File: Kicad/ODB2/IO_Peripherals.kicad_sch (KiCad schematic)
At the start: 23 parts, among them J1 Cam_Conn_01x01_Socket, J5 RFM_Conn_Coaxial, U10 W25Q512JVEIQ

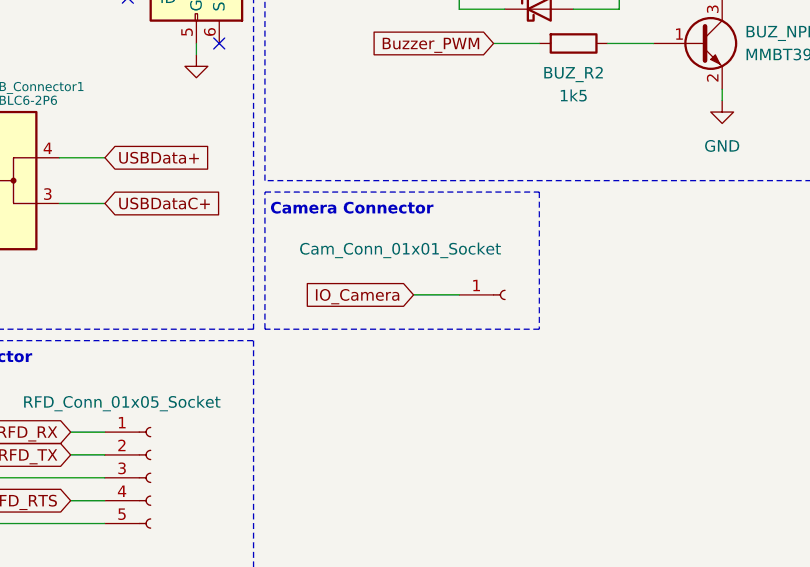
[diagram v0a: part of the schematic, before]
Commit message: fix my shit (cam io)
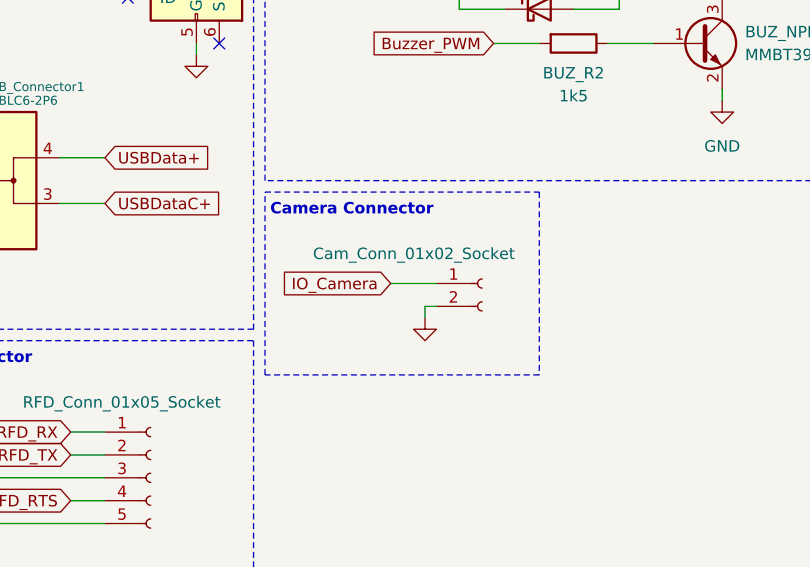
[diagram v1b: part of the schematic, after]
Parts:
- removed J1: Cam_Conn_01x01_Socket, Connector_PinHeader_2.00mm:PinHeader_1x01_P2.00mm_Vertical, symbol Connector:Conn_01x01_Socket
- added J1: Cam_Conn_01x02_Socket, Connector_PinHeader_2.00mm:PinHeader_1x02_P2.00mm_Vertical, symbol Connector:Conn_01x02_Socket
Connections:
- net GND: now also J1.2 (Pin_2)
- net IO_Camera: now also J1.1 (Pin_1)
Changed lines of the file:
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@@
 	(wire
 		(pts
+			(xy 124.46 76.2) (xy 123.19 76.2)
+		)
+		(stroke
+			(width 0)
+			(type default)
+		)
+	)
+	(wire
+		(pts
 			(xy 54.61 119.38) (xy 54.61 120.65)
 		)
@@
 	(wire
 		(pts
+			(xy 123.19 76.2) (xy 123.19 77.47)
+		)
+		(stroke
+			(width 0)
+			(type default)
+		)
+	)
+	(wire
+		(pts
 			(xy 64.77 95.25) (xy 87.63 95.25)
 		)
@@
 	(wire
 		(pts
-			(xy 121.92 74.93) (xy 127 74.93)
+			(xy 119.38 73.66) (xy 124.46 73.66)
 		)
 		(stroke
@@
 	(rectangle
 		(start 105.41 63.5)
-		(end 135.89 78.74)
+		(end 135.89 83.82)
 		(stroke
 			(width 0)
@@
 	(global_label "IO_Camera"
 		(shape input)
-		(at 121.92 74.93 180)
+		(at 119.38 73.66 180)
 		(fields_autoplaced yes)
 		(effects
@@
 		)
 		(property "Intersheetrefs" "${INTERSHEET_REFS}"
-			(at 108.8958 74.93 0)
+			(at 106.3558 73.66 0)
 			(effects
 				(font
@@
 	)
 	(symbol
-		(lib_id "Connector:Conn_01x01_Socket")
-		(at 132.08 74.93 0)
-		(unit 1)
-		(exclude_from_sim no)
-		(in_bom yes)
-		(on_board yes)
-		(dnp no)
-		(property "Reference" "J1"
-			(at 133.35 73.6599 0)
-			(effects
-				(font
-					(size 1.27 1.27)
-				)
-				(justify left)
-				(hide yes)
-			)
-		)
-		(property "Value" "Cam_Conn_01x01_Socket"
-			(at 109.22 69.85 0)
-			(effects
-				(font
-					(size 1.27 1.27)
-				)
-				(justify left)
-			)
-		)
-		(property "Footprint" "Connector_PinHeader_2.00mm:PinHeader_1x01_P2.00mm_Vertical"
-			(at 132.08 74.93 0)
-			(effects
-				(font
-					(size 1.27 1.27)
-				)
-				(hide yes)
-			)
-		)
-		(property "Datasheet" "~"
-			(at 132.08 74.93 0)
-			(effects
-				(font
-					(size 1.27 1.27)
-				)
-				(hide yes)
-			)
-		)
-		(property "Description" "Generic connector, single row, 01x01, script generated"
-			(at 132.08 74.93 0)
-			(effects
-				(font
-					(size 1.27 1.27)
-				)
-				(hide yes)
-			)
-		)
-		(pin "1"
-		)
-		(instances
-			(project ""
-				(path "/4b06c5d1-aa8b-48ed-8972-b43a60cfab78/93865dc8-71fa-4dc6-90ce-f5a9779dfd41"
-					(reference "J1")
-					(unit 1)
-				)
-			)
-		)
-	)
-	(symbol
 		(lib_id "Device:R")
 		(at 250.19 46.99 90)
@@
 	)
 	(symbol
+		(lib_id "power:GND")
+		(at 123.19 77.47 0)
+		(unit 1)
+		(exclude_from_sim no)
+		(in_bom yes)
+		(on_board yes)
+		(dnp no)
+		(fields_autoplaced yes)
+		(property "Reference" "#PWR082"
+			(at 123.19 83.82 0)
+			(effects
+				(font
+					(size 1 1)
+				)
+				(hide yes)
+			)
+		)
+		(property "Value" "GND"
+			(at 123.19 82.55 0)
+			(effects
+				(font
+					(size 1 1)
+				)
+				(hide yes)
+			)
+		)
+		(property "Footprint" ""
+			(at 123.19 77.47 0)
+			(effects
+				(font
+					(size 1 1)
+				)
+				(hide yes)
+			)
+		)
+		(property "Datasheet" ""
+			(at 123.19 77.47 0)
+			(effects
+				(font
+					(size 1 1)
+				)
+				(hide yes)
+			)
+		)
+		(property "Description" ""
+			(at 123.19 77.47 0)
+			(effects
+				(font
+					(size 1.27 1.27)
+				)
+				(hide yes)
+			)
+		)
+		(pin "1"
+		)
+		(instances
+			(project "ODB2"
+				(path "/4b06c5d1-aa8b-48ed-8972-b43a60cfab78/93865dc8-71fa-4dc6-90ce-f5a9779dfd41"
+					(reference "#PWR082")
+					(unit 1)
+				)
+			)
+		)
+	)
+	(symbol
 		(lib_id "Device:R")
 		(at 40.64 119.38 270)
@@
 					(unit 1)
 				)
+			)
+		)
+	)
+	(symbol
+		(lib_id "Connector:Conn_01x02_Socket")
+		(at 129.54 73.66 0)
+		(unit 1)
+		(exclude_from_sim no)
+		(in_bom yes)
+		(on_board yes)
+		(dnp no)
+		(property "Reference" "J1"
+			(at 130.81 73.6599 0)
+			(effects
+				(font
+					(size 1.27 1.27)
+				)
+				(justify left)
+				(hide yes)
+			)
+		)
+		(property "Value" "Cam_Conn_01x02_Socket"
+			(at 110.744 70.358 0)
+			(effects
+				(font
+					(size 1.27 1.27)
+				)
+				(justify left)
+			)
+		)
+		(property "Footprint" "Connector_PinHeader_2.00mm:PinHeader_1x02_P2.00mm_Vertical"
+			(at 129.54 73.66 0)
+			(effects
+				(font
+					(size 1.27 1.27)
+				)
+				(hide yes)
+			)
+		)
+		(property "Datasheet" "~"
+			(at 129.54 73.66 0)
+			(effects
+				(font
+					(size 1.27 1.27)
+				)
+				(hide yes)
+			)
+		)
+		(property "Description" "Generic connector, single row, 01x02, script generated"
+			(at 129.54 73.66 0)
+			(effects
+				(font
+					(size 1.27 1.27)
+				)
+				(hide yes)
+			)
+		)
+		(pin "1"
+		)
+		(pin "2"
+		)
+		(instances
+			(project ""
+				(path "/4b06c5d1-aa8b-48ed-8972-b43a60cfab78/93865dc8-71fa-4dc6-90ce-f5a9779dfd41"
+					(reference "J1")
+					(unit 1)
+				)

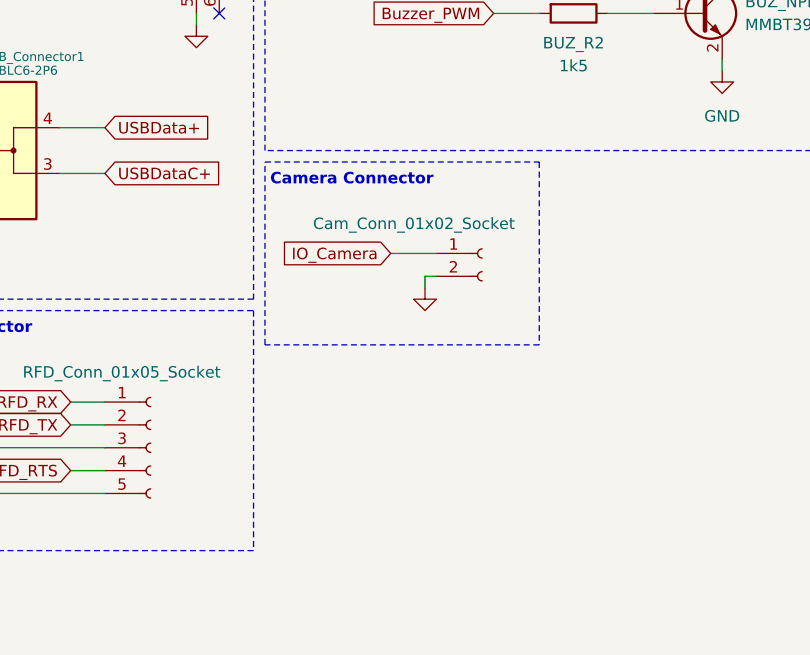
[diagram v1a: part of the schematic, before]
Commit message: ajout cam2
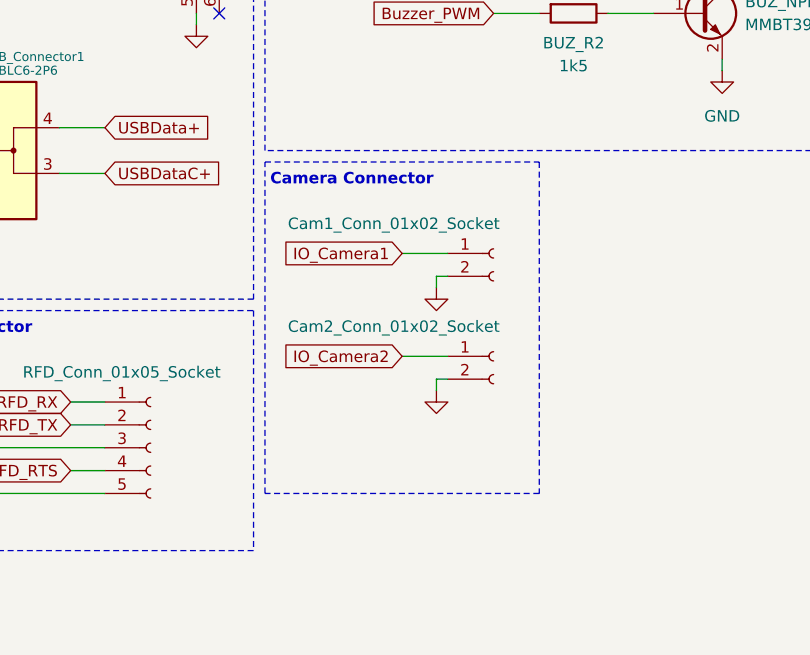
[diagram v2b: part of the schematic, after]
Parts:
- added J2: Cam2_Conn_01x02_Socket, Connector_PinHeader_2.00mm:PinHeader_1x02_P2.00mm_Vertical, symbol Connector:Conn_01x02_Socket
- J1: value Cam_Conn_01x02_Socket -> Cam1_Conn_01x02_Socket
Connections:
- net GND: now also J2.2 (Pin_2)
- net IO_Camera renamed IO_Camera1
- new net IO_Camera2: J2.1 (Pin_1)
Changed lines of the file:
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@@
 	(wire
 		(pts
+			(xy 120.65 85.09) (xy 125.73 85.09)
+		)
+		(stroke
+			(width 0)
+			(type default)
+		)
+	)
+	(wire
+		(pts
 			(xy 31.75 48.26) (xy 39.37 48.26)
 		)
@@
 	(wire
 		(pts
+			(xy 124.46 87.63) (xy 124.46 88.9)
+		)
+		(stroke
+			(width 0)
+			(type default)
+		)
+	)
+	(wire
+		(pts
+			(xy 125.73 87.63) (xy 124.46 87.63)
+		)
+		(stroke
+			(width 0)
+			(type default)
+		)
+	)
+	(wire
+		(pts
 			(xy 31.75 33.02) (xy 31.75 39.37)
 		)
@@
 	(wire
 		(pts
-			(xy 124.46 76.2) (xy 123.19 76.2)
+			(xy 125.73 76.2) (xy 124.46 76.2)
 		)
 		(stroke
@@
 	(wire
 		(pts
-			(xy 123.19 76.2) (xy 123.19 77.47)
+			(xy 124.46 76.2) (xy 124.46 77.47)
 		)
 		(stroke
@@
 	(wire
 		(pts
-			(xy 119.38 73.66) (xy 124.46 73.66)
+			(xy 120.65 73.66) (xy 125.73 73.66)
 		)
 		(stroke
@@
 	(rectangle
 		(start 105.41 63.5)
-		(end 135.89 83.82)
+		(end 135.89 100.33)
 		(stroke
 			(width 0)
@@
 		)
 	)
-	(global_label "IO_Camera"
+	(global_label "IO_Camera1"
 		(shape input)
-		(at 119.38 73.66 180)
+		(at 120.65 73.66 180)
 		(fields_autoplaced yes)
 		(effects
@@
 		)
 		(property "Intersheetrefs" "${INTERSHEET_REFS}"
-			(at 106.3558 73.66 0)
+			(at 106.4163 73.66 0)
 			(effects
 				(font
@@
 		)
 	)
+	(global_label "IO_Camera2"
+		(shape input)
+		(at 120.65 85.09 180)
+		(fields_autoplaced yes)
+		(effects
+			(font
+				(size 1.27 1.27)
+			)
+			(justify right)
+		)
+		(property "Intersheetrefs" "${INTERSHEET_REFS}"
+			(at 106.4163 85.09 0)
+			(effects
+				(font
+					(size 1.27 1.27)
+				)
+				(justify right)
+				(hide yes)
+			)
+		)
+	)
 	(global_label "SYS_SWCLK"
 		(shape input)
@@
 	(symbol
 		(lib_id "power:GND")
-		(at 123.19 77.47 0)
+		(at 124.46 77.47 0)
 		(unit 1)
 		(exclude_from_sim no)
@@
 		(fields_autoplaced yes)
 		(property "Reference" "#PWR082"
-			(at 123.19 83.82 0)
+			(at 124.46 83.82 0)
 			(effects
 				(font
@@
 		)
 		(property "Value" "GND"
-			(at 123.19 82.55 0)
+			(at 124.46 82.55 0)
 			(effects
 				(font
@@
 		)
 		(property "Footprint" ""
-			(at 123.19 77.47 0)
+			(at 124.46 77.47 0)
 			(effects
 				(font
@@
 		)
 		(property "Datasheet" ""
-			(at 123.19 77.47 0)
+			(at 124.46 77.47 0)
 			(effects
 				(font
@@
 		)
 		(property "Description" ""
-			(at 123.19 77.47 0)
+			(at 124.46 77.47 0)
 			(effects
 				(font
@@
 	)
 	(symbol
+		(lib_id "Connector:Conn_01x02_Socket")
+		(at 130.81 85.09 0)
+		(unit 1)
+		(exclude_from_sim no)
+		(in_bom yes)
+		(on_board yes)
+		(dnp no)
+		(property "Reference" "J2"
+			(at 132.08 85.0899 0)
+			(effects
+				(font
+					(size 1.27 1.27)
+				)
+				(justify left)
+				(hide yes)
+			)
+		)
+		(property "Value" "Cam2_Conn_01x02_Socket"
+			(at 107.95 81.788 0)
+			(effects
+				(font
+					(size 1.27 1.27)
+				)
+				(justify left)
+			)
+		)
+		(property "Footprint" "Connector_PinHeader_2.00mm:PinHeader_1x02_P2.00mm_Vertical"
+			(at 130.81 85.09 0)
+			(effects
+				(font
+					(size 1.27 1.27)
+				)
+				(hide yes)
+			)
+		)
+		(property "Datasheet" "~"
+			(at 130.81 85.09 0)
+			(effects
+				(font
+					(size 1.27 1.27)
+				)
+				(hide yes)
+			)
+		)
+		(property "Description" "Generic connector, single row, 01x02, script generated"
+			(at 130.81 85.09 0)
+			(effects
+				(font
+					(size 1.27 1.27)
+				)
+				(hide yes)
+			)
+		)
+		(pin "1"
+		)
+		(pin "2"
+		)
+		(instances
+			(project "ODB2"
+				(path "/4b06c5d1-aa8b-48ed-8972-b43a60cfab78/93865dc8-71fa-4dc6-90ce-f5a9779dfd41"
+					(reference "J2")
+					(unit 1)
+				)
+			)
+		)
+	)
+	(symbol
 		(lib_id "power:GND")
 		(at 223.52 99.06 0)
@@
 	)
 	(symbol
+		(lib_id "power:GND")
+		(at 124.46 88.9 0)
+		(unit 1)
+		(exclude_from_sim no)
+		(in_bom yes)
+		(on_board yes)
+		(dnp no)
+		(fields_autoplaced yes)
+		(property "Reference" "#PWR093"
+			(at 124.46 95.25 0)
+			(effects
+				(font
+					(size 1 1)
+				)
+				(hide yes)
+			)
+		)
+		(property "Value" "GND"
+			(at 124.46 93.98 0)
+			(effects
+				(font
+					(size 1 1)
+				)
+				(hide yes)
+			)
+		)
+		(property "Footprint" ""
+			(at 124.46 88.9 0)
+			(effects
+				(font
+					(size 1 1)
+				)
+				(hide yes)
+			)
+		)
+		(property "Datasheet" ""
+			(at 124.46 88.9 0)
+			(effects
+				(font
+					(size 1 1)
+				)
+				(hide yes)
+			)
+		)
+		(property "Description" ""
+			(at 124.46 88.9 0)
+			(effects
+				(font
+					(size 1.27 1.27)
+				)
+				(hide yes)
+			)
+		)
+		(pin "1"
+		)
+		(instances
+			(project "ODB2"
+				(path "/4b06c5d1-aa8b-48ed-8972-b43a60cfab78/93865dc8-71fa-4dc6-90ce-f5a9779dfd41"
+					(reference "#PWR093")
+					(unit 1)
+				)
+			)
+		)
+	)
+	(symbol
 		(lib_id "Connector:Conn_01x05_Socket")
 		(at 45.72 95.25 0)
@@
 	(symbol
 		(lib_id "Connector:Conn_01x02_Socket")
-		(at 129.54 73.66 0)
+		(at 130.81 73.66 0)
 		(unit 1)
 		(exclude_from_sim no)
@@
 		(dnp no)
 		(property "Reference" "J1"
-			(at 130.81 73.6599 0)
+			(at 132.08 73.6599 0)
 			(effects
 				(font
@@
 			)
 		)
-		(property "Value" "Cam_Conn_01x02_Socket"
-			(at 110.744 70.358 0)
+		(property "Value" "Cam1_Conn_01x02_Socket"
+			(at 107.95 70.358 0)
 			(effects
 				(font
@@
 		)
 		(property "Footprint" "Connector_PinHeader_2.00mm:PinHeader_1x02_P2.00mm_Vertical"
-			(at 129.54 73.66 0)
+			(at 130.81 73.66 0)
 			(effects
 				(font
@@
 		)
 		(property "Datasheet" "~"
-			(at 129.54 73.66 0)
+			(at 130.81 73.66 0)
 			(effects
 				(font
@@
 		)
 		(property "Description" "Generic connector, single row, 01x02, script generated"
-			(at 129.54 73.66 0)
+			(at 130.81 73.66 0)
 			(effects
 				(font
